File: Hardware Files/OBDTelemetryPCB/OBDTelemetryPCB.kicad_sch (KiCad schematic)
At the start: 10 parts, among them J1 InputSocket, J2 USB_C_Receptacle_USB2.0_14P, U1 ESP32-WROOM-32E, U2 SN65HVD230, U3 CP2102N-Axx-xQFN20, U4 TLV76133DCY

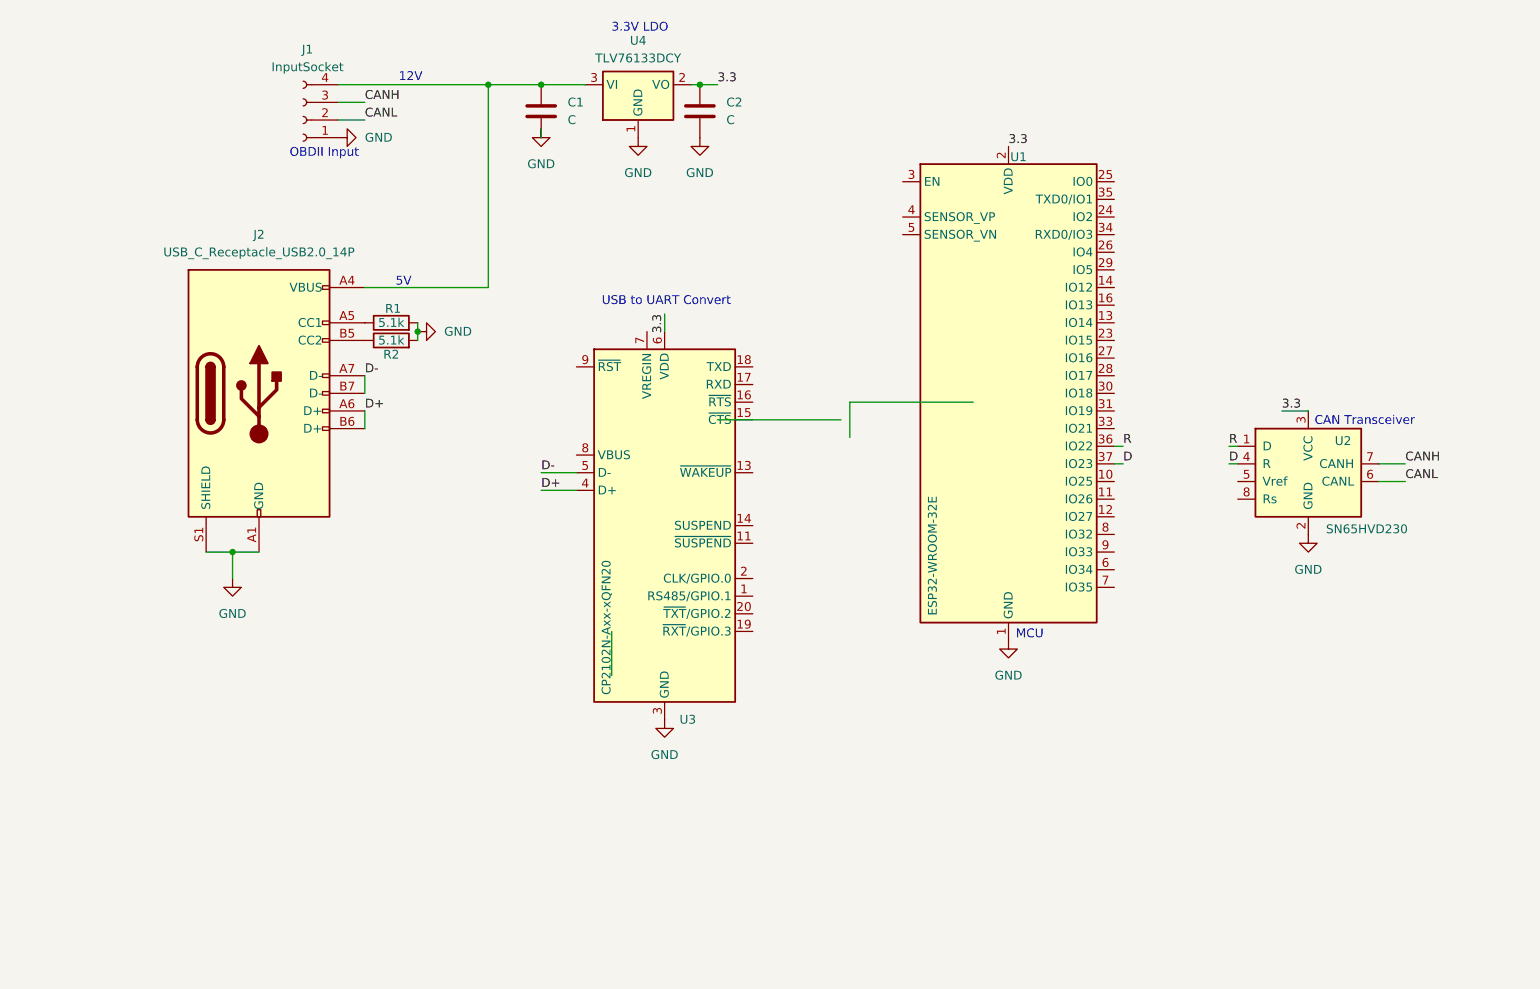
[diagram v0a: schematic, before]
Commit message: Updated PCB
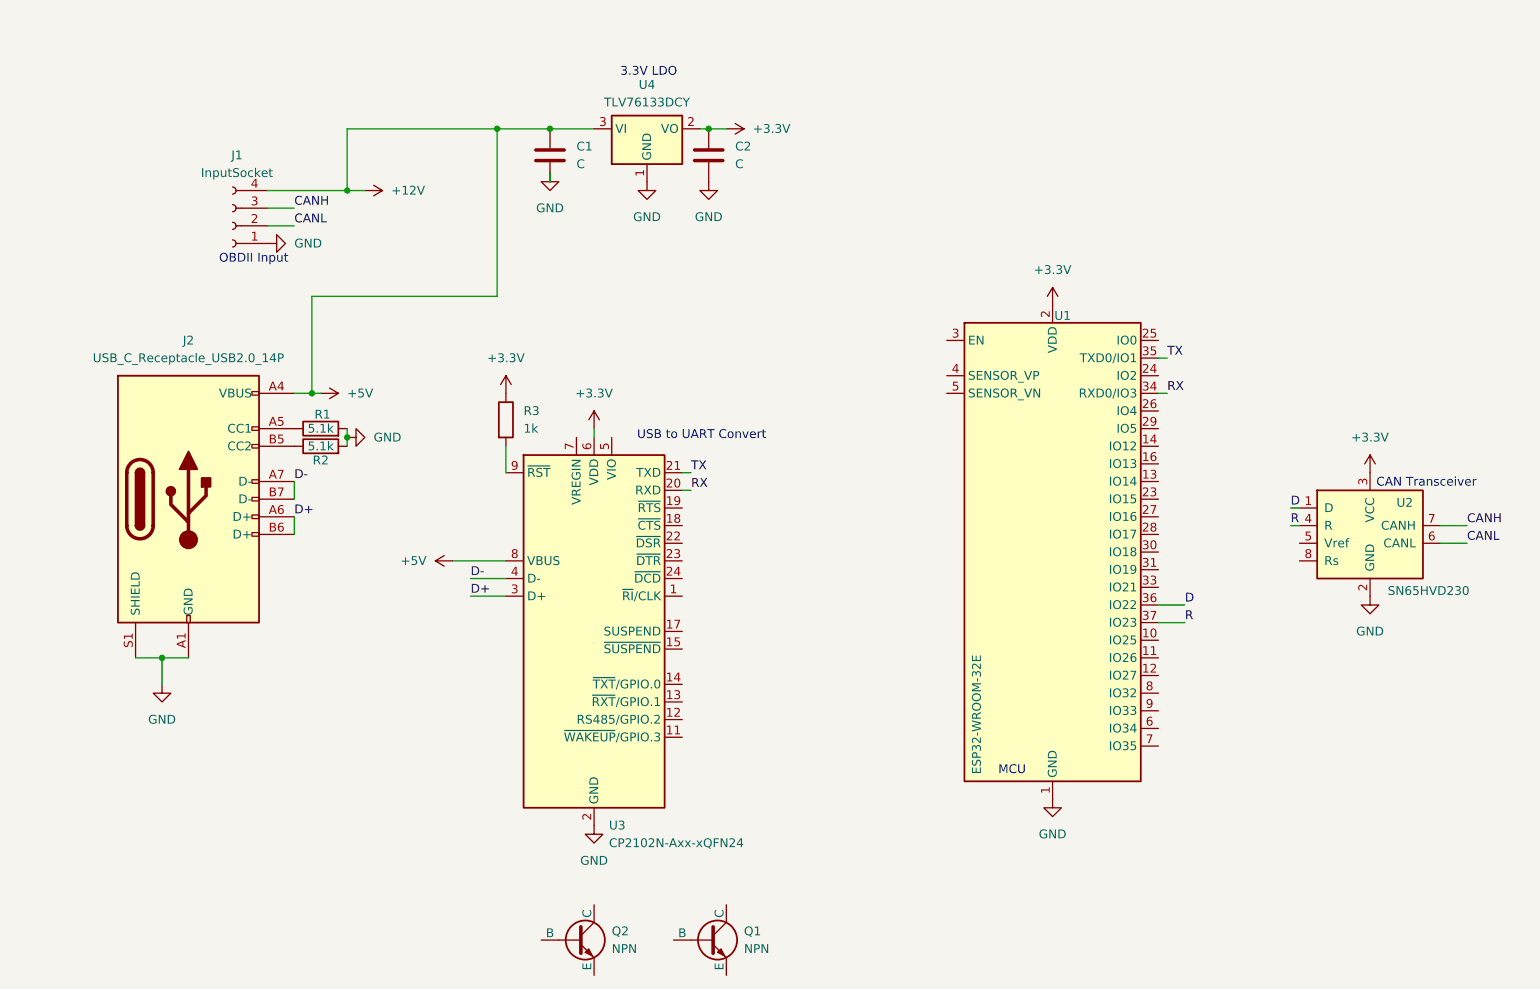
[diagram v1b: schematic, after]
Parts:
- removed U3: CP2102N-Axx-xQFN20, Package_DFN_QFN:SiliconLabs_QFN-20-1EP_3x3mm_P0.5mm_EP1.8x1.8mm, symbol Interface_USB:CP2102N-Axx-xQFN20
- added Q1, Q2: NPN, symbol Simulation_SPICE:NPN
- added R3: 1k, symbol Device:R
- added U3: CP2102N-Axx-xQFN24, Package_DFN_QFN:QFN-24-1EP_4x4mm_P0.5mm_EP2.6x2.6mm, symbol Interface_USB:CP2102N-Axx-xQFN24
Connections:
- net D: now also U1.36 (IO22), U2.1 (D); no longer U1.37 (IO23), U2.4 (R)
- net D+: now also U3.3 (D+)
- net D-: now also U3.4 (D-)
- net GND: now also U3.2 (GND), U3.25 (GND)
- net R: now also U1.37 (IO23), U2.4 (R); no longer U1.36 (IO22), U2.1 (D)
- net RX: now reaches U1.34 (RXD0/IO3)
- net RX: now also U3.20 (RXD)
- net TX: now reaches U1.35 (TXD0/IO1)
- net TX: now also U3.21 (TXD)
- net +12V: now reaches C1.1, J1.4 (Pin_4), J2.A4 (VBUS), J2.A9 (VBUS), J2.B4 (VBUS), J2.B9 (VBUS), U4.3 (VI)
- net +12V: now also U3.8 (VBUS)
- net 3.3 renamed +3.3V
- net +3.3V: now also R3.1, U3.6 (VDD)
- new net: R3.2, U3.9 (~{RST})
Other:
- note removed: "12V"
- note removed: "5V"
- moved on the sheet: C1, C2, J1, J2, R1, R2, U1, U2, U4

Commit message: Completed v1 of hardware
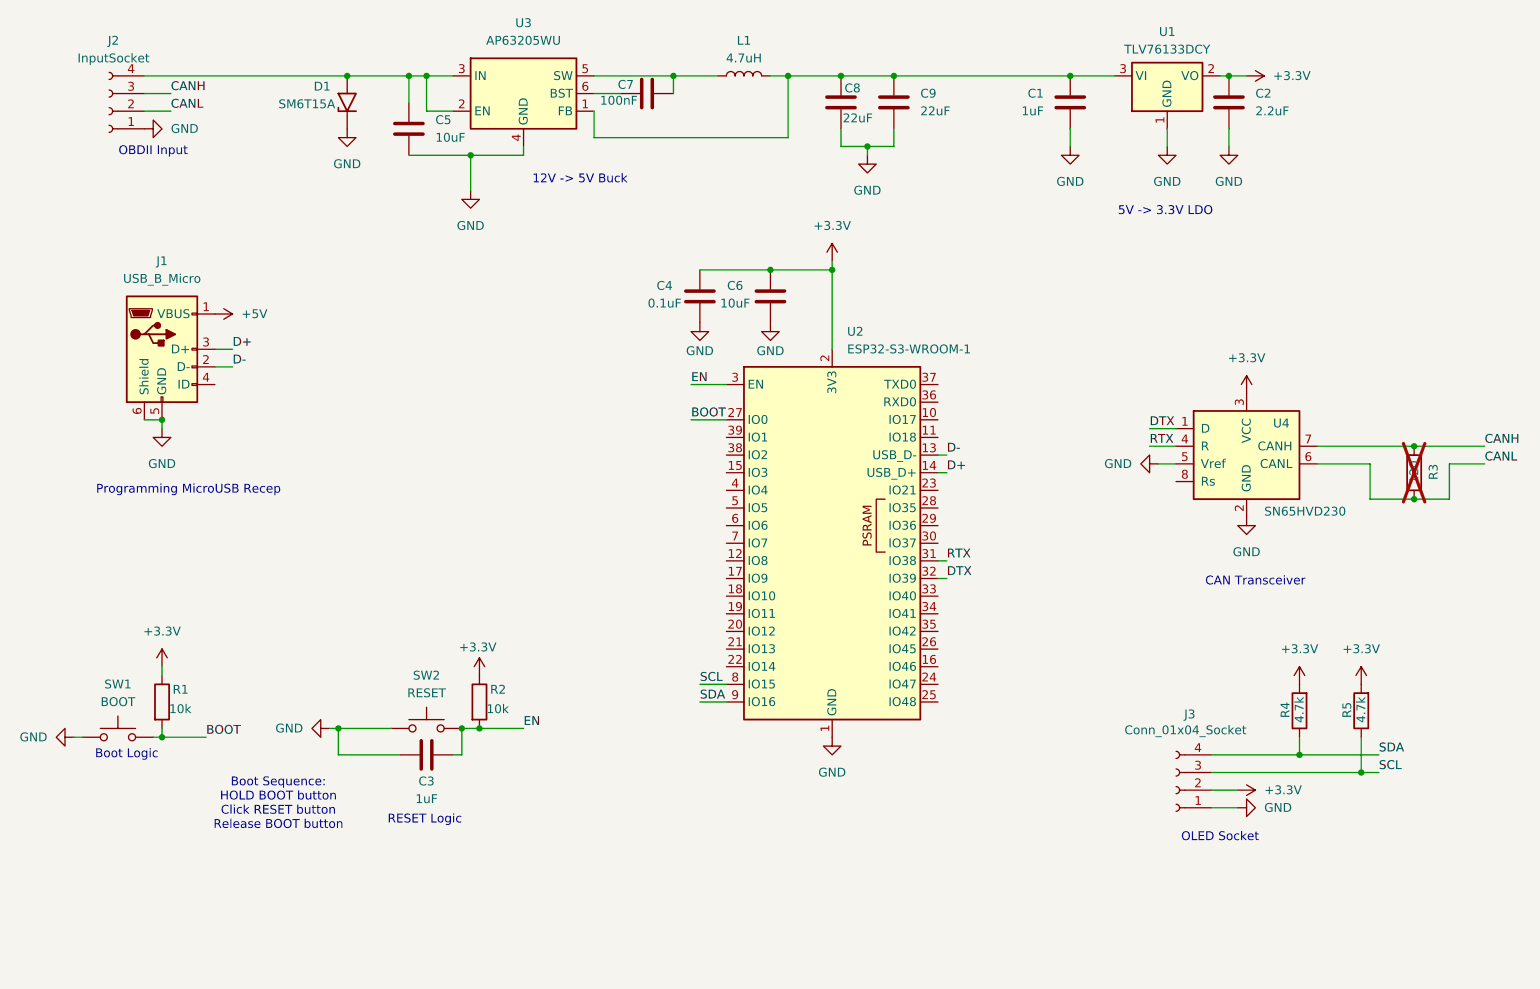
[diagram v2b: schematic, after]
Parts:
- removed J2: USB_C_Receptacle_USB2.0_14P, symbol Connector:USB_C_Receptacle_USB2.0_14P
- removed Q1, Q2: NPN, symbol Simulation_SPICE:NPN
- removed U1: ESP32-WROOM-32E, RF_Module:ESP32-WROOM-32D, symbol RF_Module:ESP32-WROOM-32E
- removed U3: CP2102N-Axx-xQFN24, Package_DFN_QFN:QFN-24-1EP_4x4mm_P0.5mm_EP2.6x2.6mm, symbol Interface_USB:CP2102N-Axx-xQFN24
- added C3: 1uF, Capacitor_SMD:C_0603_1608Metric, symbol Device:C
- added C4: 0.1uF, Capacitor_SMD:C_0603_1608Metric, symbol Device:C
- added C5, C6: 10uF, Capacitor_SMD:C_0603_1608Metric, symbol Device:C
- added C7: 100nF, Capacitor_SMD:C_0603_1608Metric, symbol Device:C
- added C8, C9: 22uF, Capacitor_SMD:C_0603_1608Metric, symbol Device:C
- added D1: SM6T15A, Diode_SMD:D_SOD-123, symbol Diode:SM6T15A
- added J1: USB_B_Micro, Connector_USB:USB_Micro-AB_Molex_47590-0001, symbol Connector:USB_B_Micro
- added J3: Conn_01x04_Socket, Connector_PinHeader_2.54mm:PinHeader_1x04_P2.54mm_Vertical, symbol Connector:Conn_01x04_Socket
- added L1: 4.7uH, Resistor_SMD:R_0201_0603Metric, symbol Device:L
- added R4, R5: 4.7k, Resistor_SMD:R_0201_0603Metric, symbol Device:R
- added SW1: BOOT, Button_Switch_SMD:SW_Tactile_SPST_NO_Straight_CK_PTS636Sx25SMTRLFS, symbol Switch:SW_Push
- added SW2: RESET, Button_Switch_SMD:SW_Tactile_SPST_NO_Straight_CK_PTS636Sx25SMTRLFS, symbol Switch:SW_Push
- added U2: ESP32-S3-WROOM-1, RF_Module:ESP32-S3-WROOM-1, symbol RF_Module:ESP32-S3-WROOM-1
- added U3: AP63205WU, Package_TO_SOT_SMD:TSOT-23-6, symbol Regulator_Switching:AP63205WU
- C1: value C -> 1uF; footprint (none) -> Capacitor_SMD:C_0603_1608Metric
- C2: value C -> 2.2uF; footprint (none) -> Capacitor_SMD:C_0603_1608Metric
- R1, R2: value 5.1k -> 10k; footprint (none) -> Resistor_SMD:R_0201_0603Metric
- R3: value 1k -> 120; footprint (none) -> Resistor_SMD:R_0201_0603Metric; now not fitted
- renumbered J1 to J2, U4 to U1, U2 to U4
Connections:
- net +3.3V: now also R1.1, R2.1, C4.1, C6.1, J3.2 (Pin_2), R4.2, R5.2, U2.2 (3V3); no longer R3.1
- net CANH: now also R3.2
- net CANL: now also R3.1
- net D+: now also J1.3 (D+), U2.14 (USB_D+)
- net D-: now also J1.2 (D-), U2.13 (USB_D-)
- net GND: now also U4.5 (Vref), C3.1, C4.2, C5.2, C6.2, C8.1, C9.1, D1.1 (A1), J1.5 (GND), J1.6 (Shield), J3.1 (Pin_1), SW1.1, SW2.1, U2.1 (GND), U2.40 (GND), U2.41 (GND), U3.4 (GND); no longer R1.2, R2.2
- net +12V: no longer names the net of C1.1, U1.3 (VI)
- net +12V: now also C8.2, C9.2, L1.2, U3.1 (FB); no longer J2.4 (Pin_4)
- net D renamed DTX
- net DTX: now also U2.32 (IO39)
- net R renamed RTX
- net RTX: now also U2.31 (IO38)
- new net: C5.1, D1.2 (A2), J2.4 (Pin_4), U3.2 (EN), U3.3 (IN)
- new net: C7.1, L1.1, U3.5 (SW)
- new net: C7.2, U3.6 (BST)
- new net +5V: J1.1 (VBUS)
- new net BOOT: R1.2, SW1.2, U2.27 (IO0)
- new net EN: C3.2, R2.2, SW2.2, U2.3 (EN)
- new net SCL: J3.3 (Pin_3), R5.1, U2.8 (IO15)
- new net SDA: J3.4 (Pin_4), R4.1, U2.9 (IO16)
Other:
- note added: "12V -> 5V Buck"
- note added: "5V -> 3.3V LDO"
- note added: "Boot Logic"
- note added: "Boot Sequence: HOLD BOOT button Click RESET button Release BOOT button"
- note added: "OLED Socket"
- note added: "Programming MicroUSB Recep"
- note added: "RESET Logic"
- note removed: "3.3V LDO"
- note removed: "MCU"
- note removed: "USB to UART Convert"
- moved on the sheet: C1, C2, J2, U1, U4
